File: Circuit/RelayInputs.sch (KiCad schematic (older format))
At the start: 24 parts, among them U301 LTV-817, U302 LTV-817, U303 LTV-817, U304 LTV-817, U305 LTV-817, U306 LTV-817, U307 LTV-817, U308 LTV-817

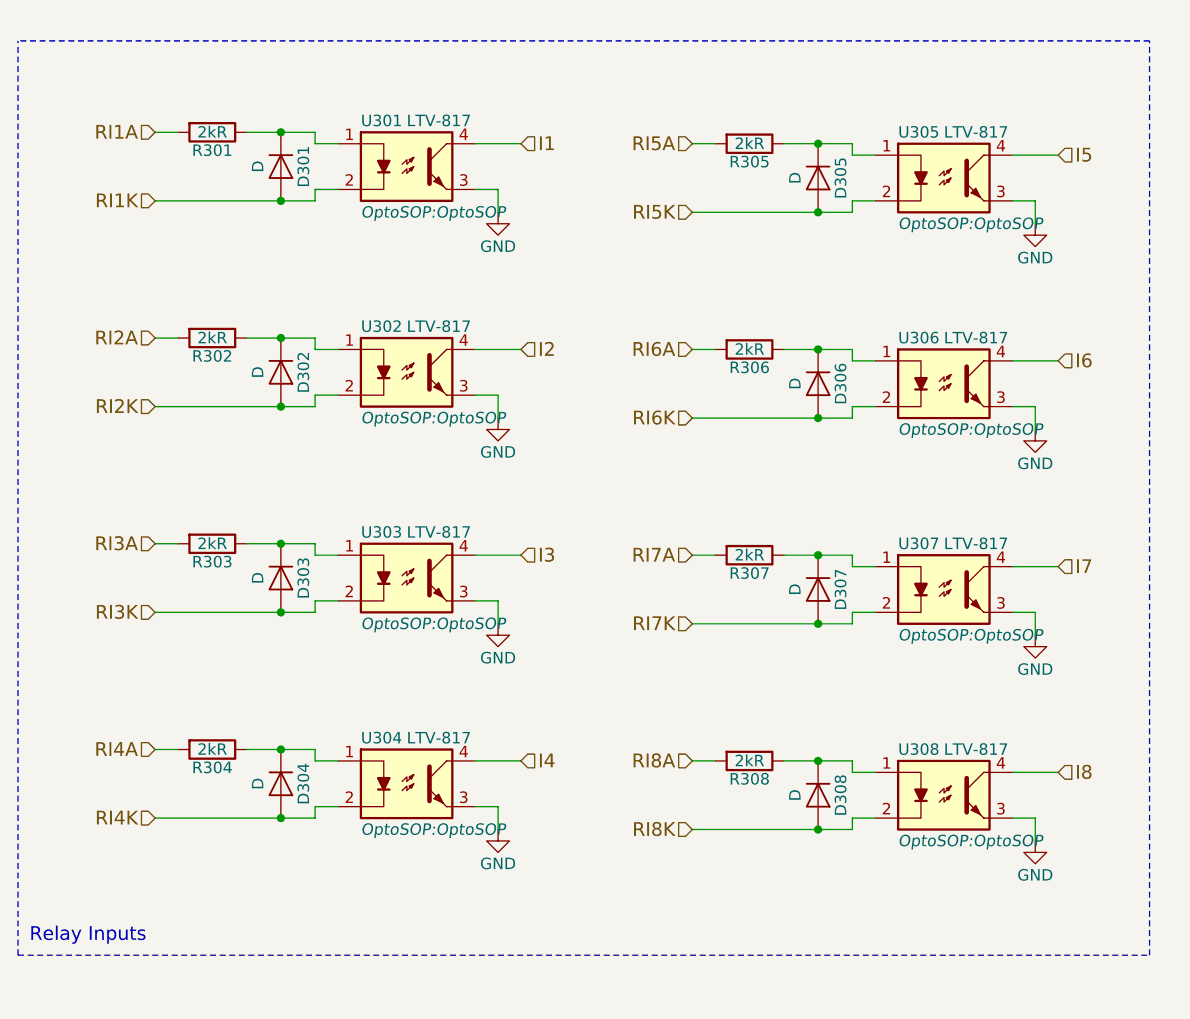
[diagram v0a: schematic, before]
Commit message: PCB. Pours mostly complete. Almost done?
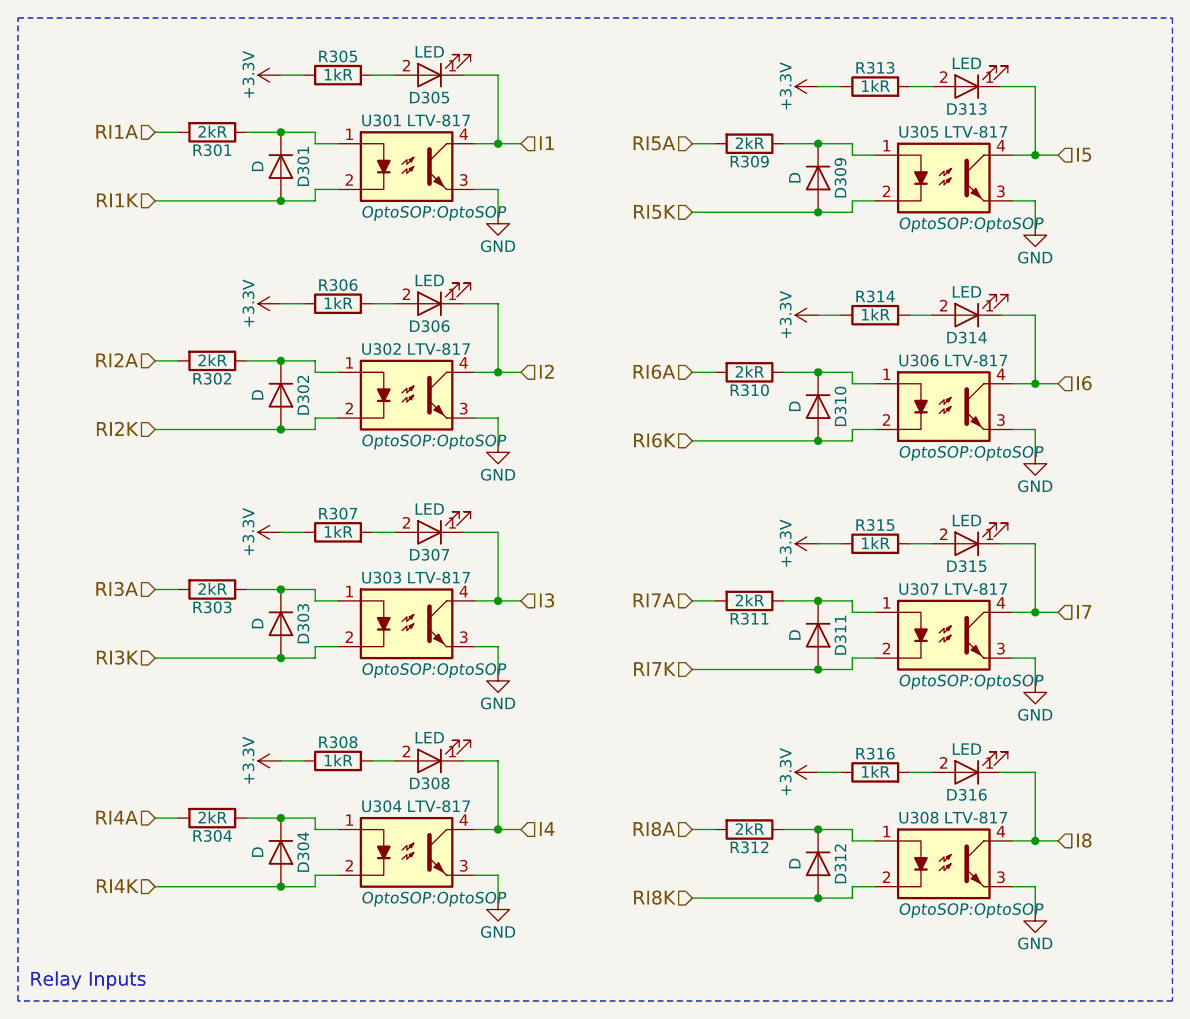
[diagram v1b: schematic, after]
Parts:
- added D305, D306, D307, D308, D313, D314, D315, D316: LED, Capacitors_SMD:C_0805, symbol LED
- added R305, R306, R307, R308, R313, R314, R315, R316: 1kR, Resistors_SMD:R_0805, symbol R
- renumbered D305 to D309, D306 to D310, D307 to D311, D308 to D312, R305 to R309, R306 to R310, R307 to R311, R308 to R312
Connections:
- net I1: now also D305.1 (K)
- net I2: now also D306.1 (K)
- net I3: now also D307.1 (K)
- net I4: now also D308.1 (K)
- net I5: now also D313.1 (K)
- net I6: now also D314.1 (K)
- net I7: now also D315.1 (K)
- net I8: now also D316.1 (K)
- new net: D305.2 (A), R305.2
- new net: D307.2 (A), R307.2
- new net: D306.2 (A), R306.2
- new net: D308.2 (A), R308.2
- new net: D313.2 (A), R313.2
- new net: D314.2 (A), R314.2
- new net: D315.2 (A), R315.2
- new net: D316.2 (A), R316.2
- new net +3V3: R305.1, R306.1, R307.1, R308.1, R313.1, R314.1, R315.1, R316.1
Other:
- moved on the sheet: D302, D303, D304, D310, D311, D312, R302, R303, R304, R310, R311, R312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
